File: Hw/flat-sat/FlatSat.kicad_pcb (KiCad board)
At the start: 4 copper layers, 48 x 32 mm, 106 parts, among them J1 Antenna, J2 Antenna, J3 periphs, J4 SWD, P1 USB_C_Plug_USB2.0, U1 TLV75733PDBVR, U10 LIS2DH, U11 BME280 /BMP280, U2 0900FM15D0039, U3 PE42421, U4 SX1262IMLTRT, U5 W25Q16JV, U6 0900FM15D0039, U7 PE42421, U8 SX1262IMLTRT, U9 RP2040, Y1 32Mhz, Y2 32Mhz, Y3 12MHz

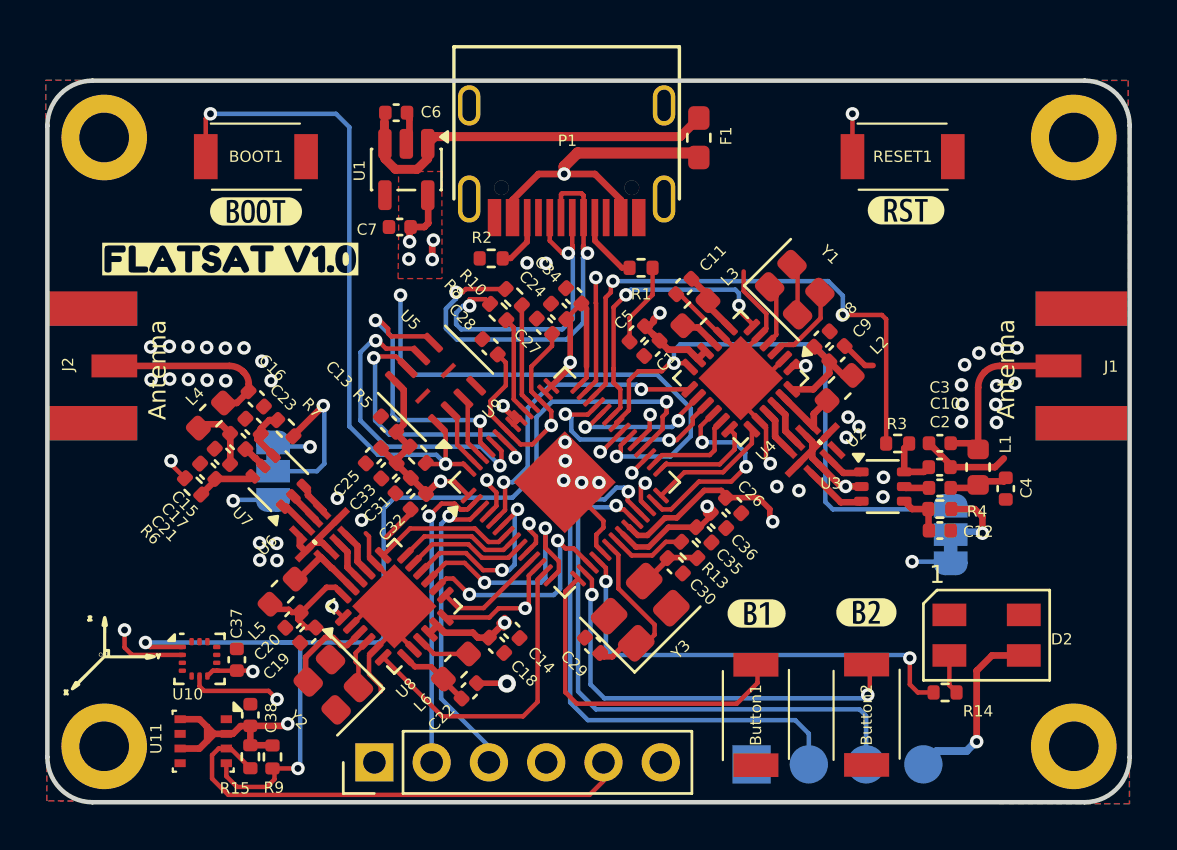
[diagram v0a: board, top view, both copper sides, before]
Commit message: feat(Hw):LC_Layout_Updated
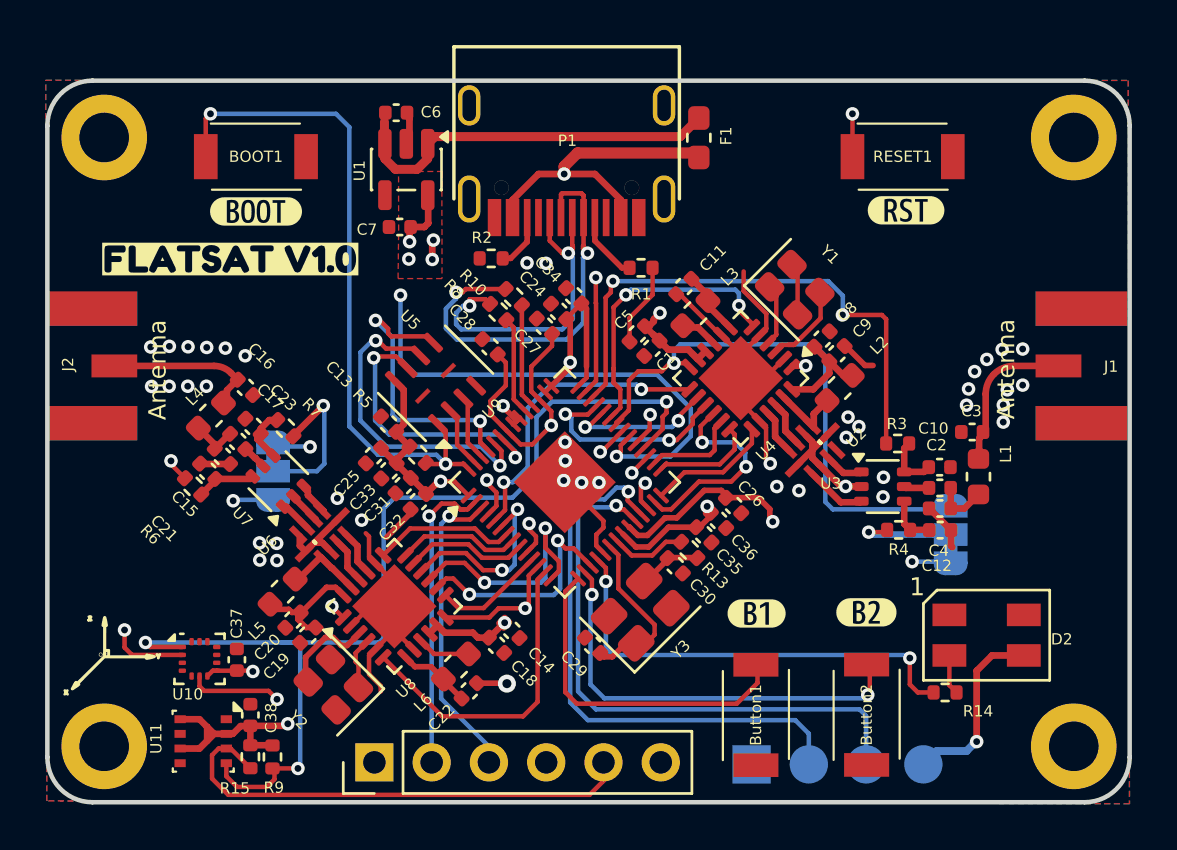
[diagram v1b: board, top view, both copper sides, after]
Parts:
- moved C4 3.05 mm to (118.3, 114.0), turned to 180 degrees
- moved R4 2.05 mm to (116.5, 114.9), turned to 180 degrees
- moved C3 1.52 mm to (119.7, 110.6)
- moved C16 0.70 mm to (87.5, 108.6)
- moved L1 0.42 mm to (120.0, 112.6)
- turned C17 to -45 degrees
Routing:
- net Net-(J1-In): track 8.18 -> 6.94 mm
- net Net-(C15-Pad2): track 3.28 -> 2.18 mm
- net Net-(J2-In): track 8.05 -> 6.98 mm
- net Net-(JP1-C): track 3.74 -> 4.54 mm
- net GND: track 62.2 -> 62.0 mm, vias 47 -> 43
